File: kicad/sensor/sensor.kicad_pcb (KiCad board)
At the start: 2 copper layers, 6 parts, among them J1 CONN, U1 150, U2 152, U3 153, U4 156, U5 155

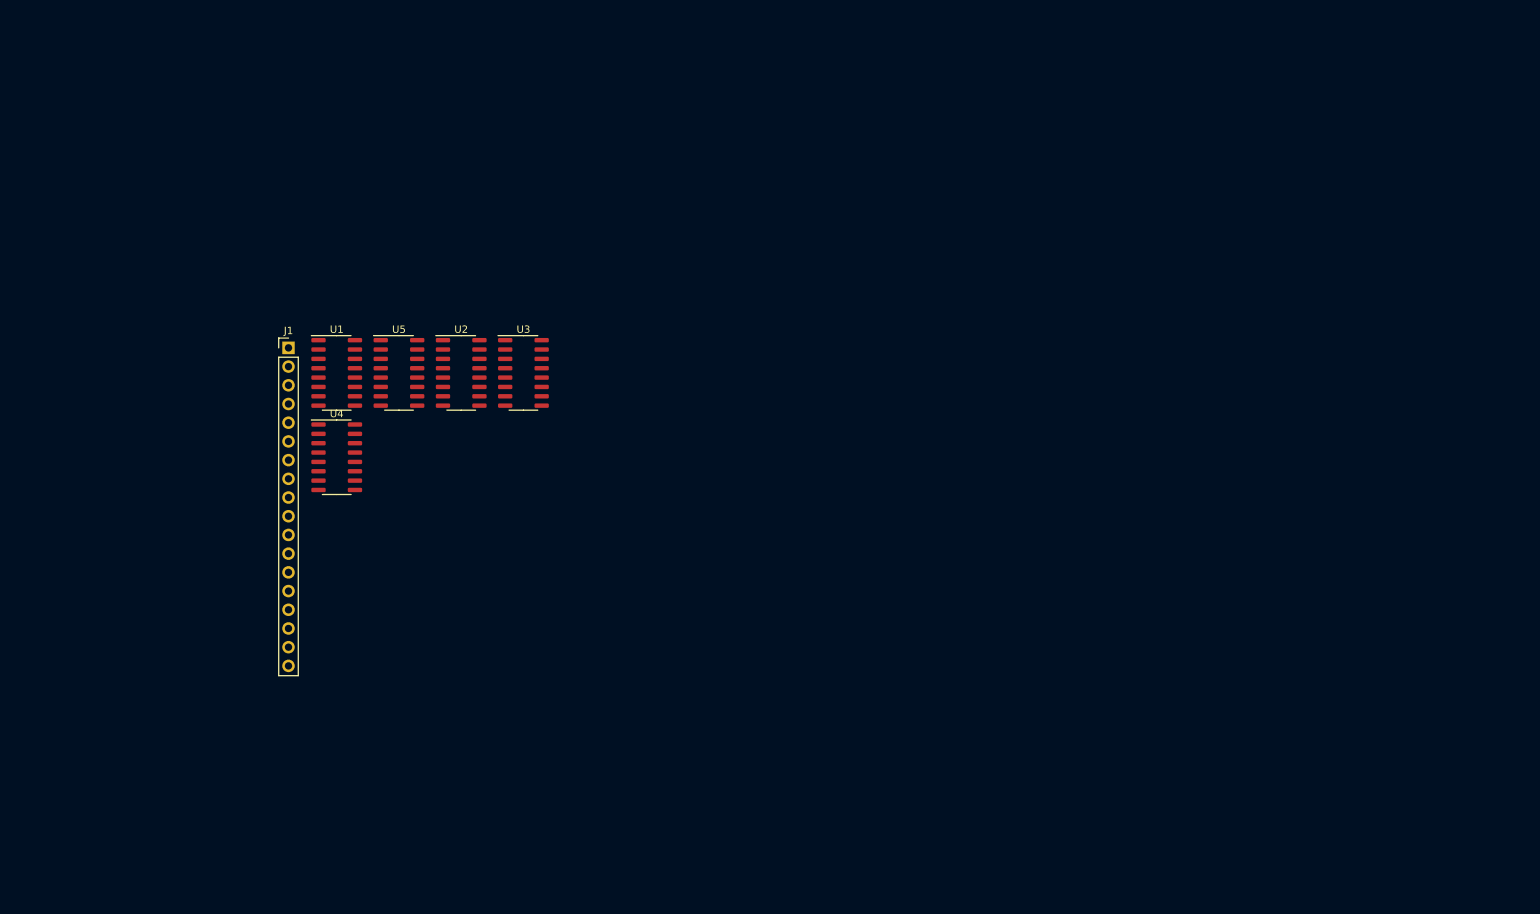
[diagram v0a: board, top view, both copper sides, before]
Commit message: add kicad plugin
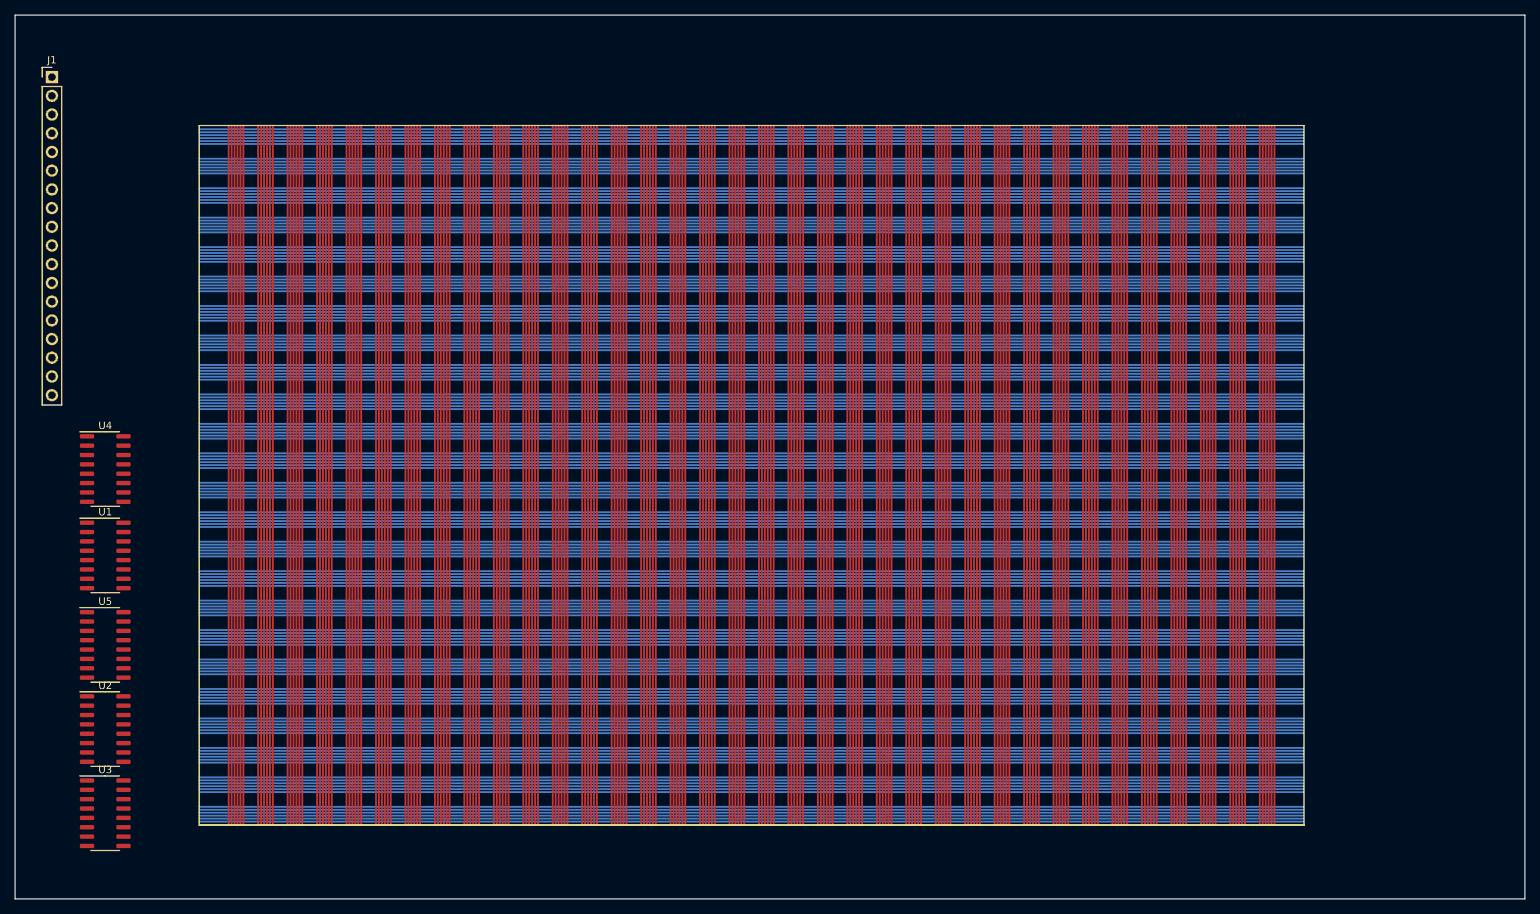
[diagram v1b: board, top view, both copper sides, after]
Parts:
- moved U3 82.5 mm to (62.2, 138.4)
- moved U2 68.4 mm to (62.2, 126.9)
- moved U5 54.4 mm to (62.2, 115.5)
- moved J1 48.8 mm to (55.0, 38.4)
- moved U1 40.0 mm to (62.2, 103.4)
- moved U4 31.5 mm to (62.2, 91.6)
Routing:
- net (no net): track 0.00 -> 42120.0 mm
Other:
- board outline added: 205 x 120 mm
